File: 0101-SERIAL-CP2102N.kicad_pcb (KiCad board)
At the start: 2 copper layers, 19.6 x 19.6 mm, 2 parts

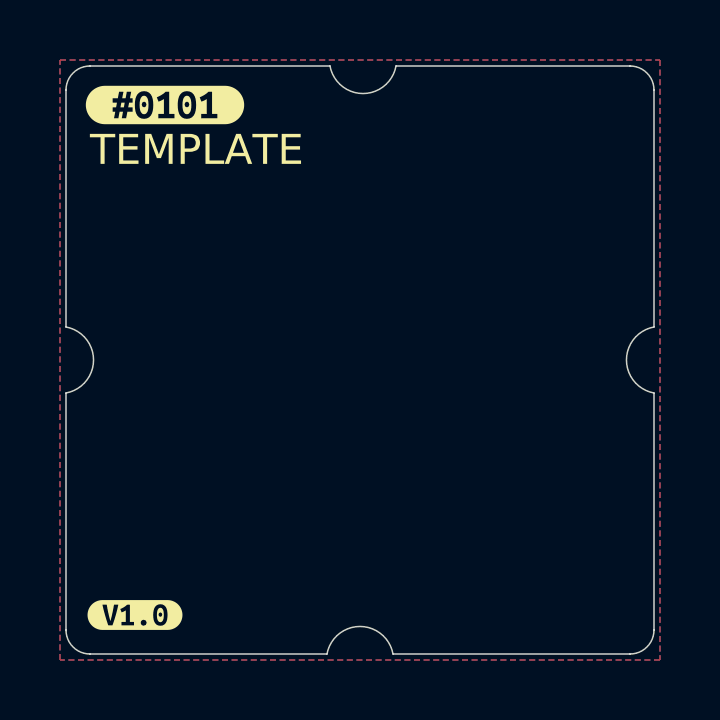
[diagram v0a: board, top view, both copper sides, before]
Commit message: Done PCB
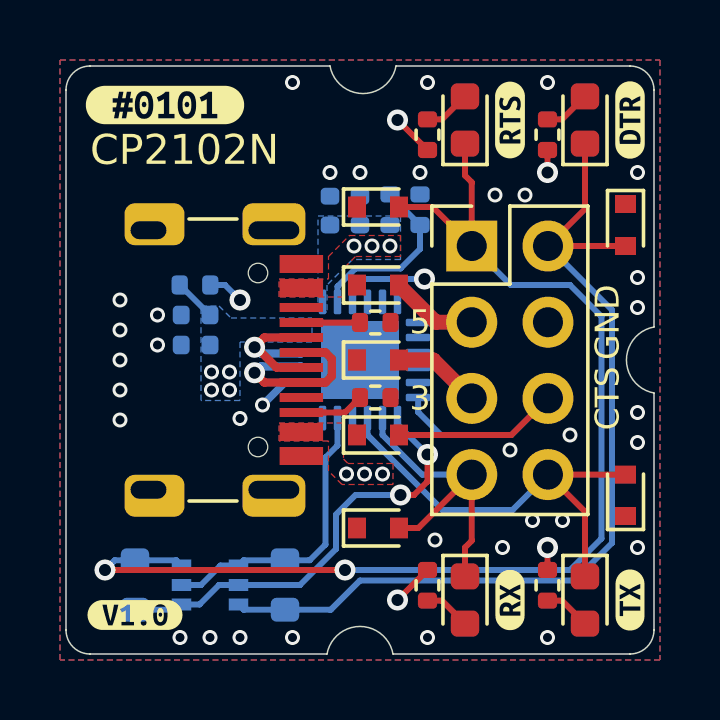
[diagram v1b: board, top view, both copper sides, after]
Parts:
- added C1: 4.7uF, Capacitor_SMD:C_0402_1005Metric, B.Cu at (104.5, 108.5)
- added C2: 4.7uF, Capacitor_SMD:C_0402_1005Metric, B.Cu at (110.0, 105.0)
- added C3: 0.1uF, Capacitor_SMD:C_0402_1005Metric, B.Cu at (104.5, 109.5)
- added C4: 0.1uF, Capacitor_SMD:C_0402_1005Metric, B.Cu at (109.0, 105.0)
- added D1: LED_YEL, LED_SMD:LED_0603_1608Metric, F.Cu at (117.5, 118.0)
- added D10: LESD5Z5.0CT1G, Diode_SMD:D_SOD-523, F.Cu at (118.8, 105.5)
- added D11: LESD5Z5.0CT1G, Diode_SMD:D_SOD-523, F.Cu at (110.6, 112.5)
- added D2: LED_YEL, LED_SMD:LED_0603_1608Metric, F.Cu at (113.5, 118.0)
- added D3: LED_BLU, LED_SMD:LED_0603_1608Metric, F.Cu at (113.5, 102.0)
- added D4: LED_RED, LED_SMD:LED_0603_1608Metric, F.Cu at (117.5, 102.0)
- added D5: LESD5Z5.0CT1G, Diode_SMD:D_SOD-523, F.Cu at (110.6, 107.5)
- added D6: LESD5Z5.0CT1G, Diode_SMD:D_SOD-523, F.Cu at (110.6, 110.0)
- added D7: LESD5Z5.0CT1G, Diode_SMD:D_SOD-523, F.Cu at (118.8, 114.5)
- added D8: LESD5Z5.0CT1G, Diode_SMD:D_SOD-523, F.Cu at (110.6, 115.6)
- added D9: LESD5Z5.0CT1G, Diode_SMD:D_SOD-523, F.Cu at (110.6, 104.9)
- added J1: USB-C, JLC-SMT:HRO_TYPE-C-31-M-12, F.Cu at (104.0, 110.0)
- added J2: Conn_02x04_Odd_Even, Connector_PinHeader_2.54mm:PinHeader_2x04_P2.54mm_Vertical, F.Cu at (113.7, 106.2)
- added Q1: DDC114TH, Package_TO_SOT_SMD:SOT-363_SC-70-6, B.Cu at (105.0, 117.5)
- added R1: 22.1K, Resistor_SMD:R_0402_1005Metric, B.Cu at (111.0, 105.0)
- added R12: 1.5K, Resistor_SMD:R_0402_1005Metric, F.Cu at (116.2, 117.5)
- added R13: 1.5K, Resistor_SMD:R_0402_1005Metric, F.Cu at (112.2, 117.5)
- added R14: 1.5K, Resistor_SMD:R_0402_1005Metric, F.Cu at (112.2, 102.5)
- added R15: 1.5K, Resistor_SMD:R_0402_1005Metric, F.Cu at (116.2, 102.5)
- added R2: 47.5K, Resistor_SMD:R_0402_1005Metric, B.Cu at (112.0, 105.0)
- added R3: 1K, Resistor_SMD:R_0402_1005Metric, B.Cu at (104.5, 107.5)
- added R4: 5.1K, Resistor_SMD:R_0402_1005Metric, F.Cu at (110.5, 108.8)
- added R5: 5.1K, Resistor_SMD:R_0402_1005Metric, F.Cu at (110.5, 111.2)
- added R8: 0R(NC), Resistor_SMD:R_0603_1608Metric, B.Cu at (107.5, 117.5)
- added R9: 0R(NC), Resistor_SMD:R_0603_1608Metric, B.Cu at (102.5, 117.5)
- added U1: CP2102N-A02-GQFN24, Package_DFN_QFN:QFN-24-1EP_4x4mm_P0.5mm_EP2.6x2.6mm, B.Cu at (110.0, 110.0)
- added kibuzzard-63353A29: G***, kibuzzard-63353A29, F.Cu at (115.0, 102.0)
- added kibuzzard-63353A37: G***, kibuzzard-63353A37, F.Cu at (119.0, 102.0)
- added kibuzzard-63395349: G***, kibuzzard-63395349, F.Cu at (115.0, 118.0)
- added kibuzzard-6339534D: G***, kibuzzard-6339534D, F.Cu at (119.0, 118.0)
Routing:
- net VDD: track 0.00 -> 45.4 mm, vias 0 -> 8
- net /RTS/BOOT: track 0.00 -> 38.9 mm, vias 0 -> 2
- net /DTR/RESET: track 0.00 -> 30.7 mm
- net /RTS: track 0.00 -> 14.7 mm, vias 0 -> 2
- net /TXD: track 0.00 -> 14.6 mm
- net Net-(R3-Pad2): track 0.00 -> 13.9 mm, vias 0 -> 2
- net /CTS: track 0.00 -> 11.1 mm
- net /RXD: track 0.00 -> 10.7 mm
- net /DTR: track 0.00 -> 9.74 mm
- net /D+: track 0.00 -> 6.16 mm, vias 0 -> 1
- net Net-(R1-Pad2): track 0.00 -> 6.01 mm
- net /D-: track 0.00 -> 5.21 mm, vias 0 -> 1
- net GND: track 0.00 -> 3.87 mm, vias 0 -> 35
- net VBUS: track 0.00 -> 2.94 mm, vias 0 -> 6
- net Net-(J1-PadB5): track 0.00 -> 2.16 mm
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- added copper zone on B.Cu, net GND
- added copper zone on F.Cu, net GND
- added copper zone on In1.Cu, net GND
- added copper zone on In2.Cu, net GND
- added copper zone on B.Cu, net VBUS
- added copper zone on F.Cu, net VBUS
- added copper zone on In1.Cu, net VBUS
- added copper zone on In2.Cu, net VBUS
- added copper zone on B.Cu, net VDD
- added copper zone on In1.Cu, net VDD
- removed copper zone on B.Cu, net (none)
- removed copper zone on F.Cu, net (none)
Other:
- outline, holes or cut-outs redrawn
- copper layers 2 -> 4
- board text added: "3"
- board text added: "5"
- board text added: "CP2102N"
- board text added: "CTS"
- board text added: "GND"
- board text removed: "TEMPLATE"
